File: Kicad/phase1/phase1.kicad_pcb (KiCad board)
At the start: 2 copper layers, 150.1 x 100.1 mm, 50 parts, among them Q1 IRFZ46N, Q2 IRFZ46N, Q3 IRFZ46N, Q4 IRFZ46N, Q5 IRFZ46N, Q6 IRFZ46N, U1 IR2102, U2 IR2102, U3 IR2102, U4 ACS712, U5 7805, U6 Atmega328P, Y1 Crystal

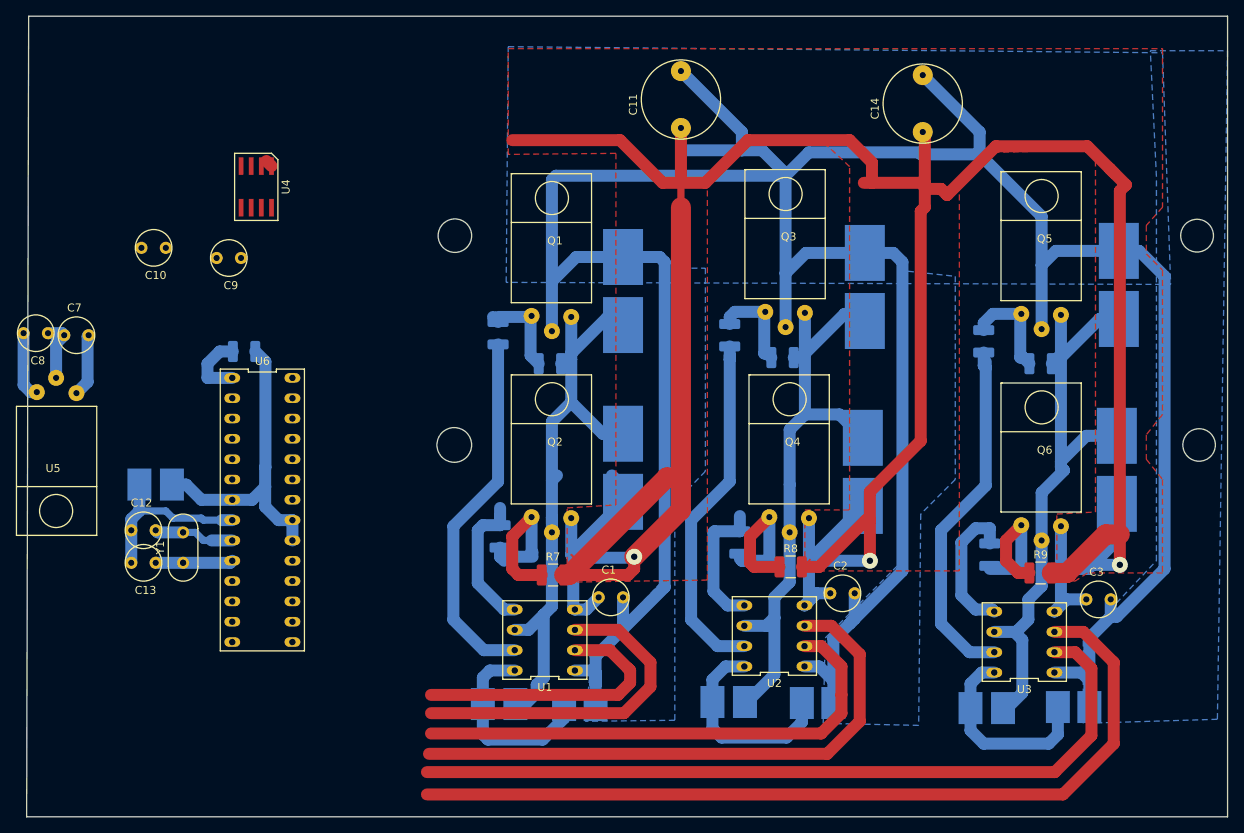
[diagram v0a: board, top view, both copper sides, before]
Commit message: .
.
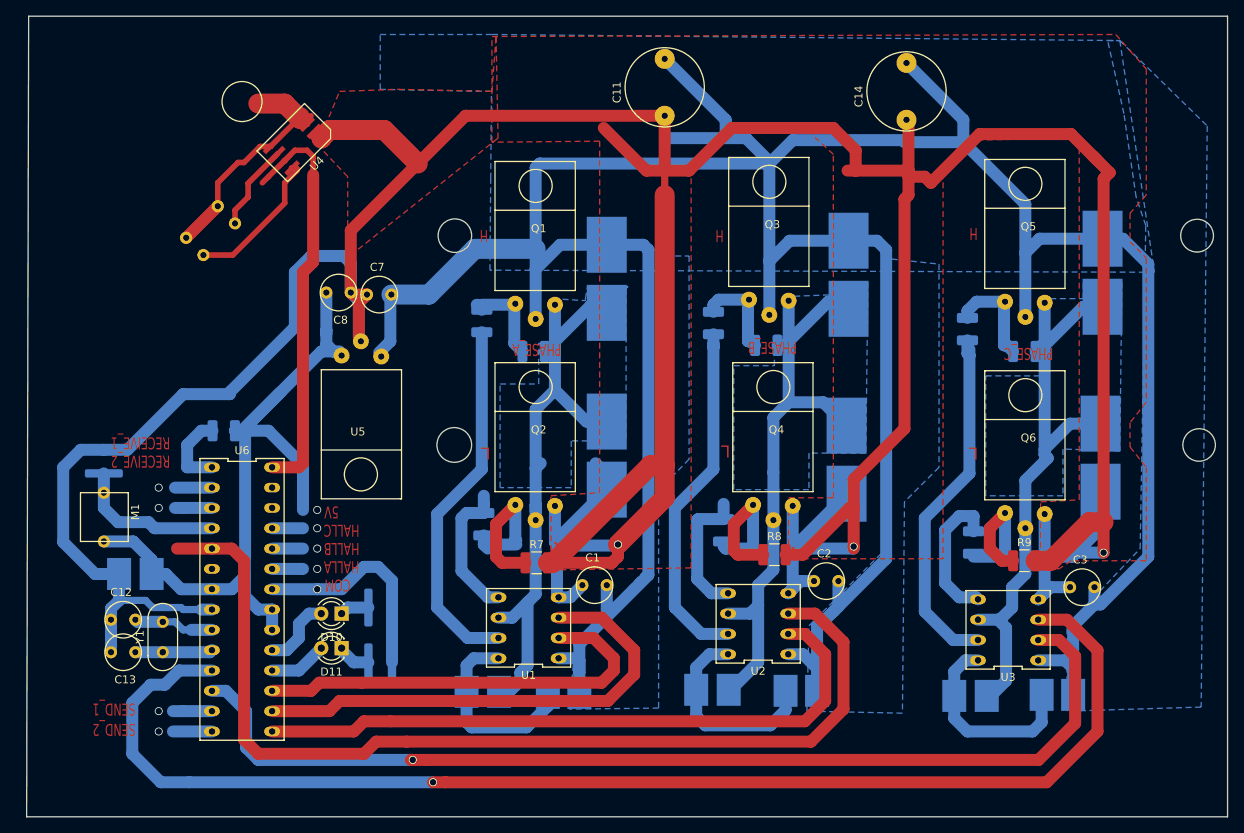
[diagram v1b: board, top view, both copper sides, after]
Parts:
- added D10: LED, LED_THT:LED_D3.0mm, F.Cu at (121.9, 87.9)
- added D11: LED, LED_THT:LED_D3.0mm, F.Cu at (121.9, 92.2)
- added M1: button, phase1:button, F.Cu at (92.2, 75.7)
- added R14: 400, Resistor_SMD:R_1218_3246Metric, B.Cu at (126.7, 87.1)
- added R15: 400, Resistor_SMD:R_1218_3246Metric, B.Cu at (126.7, 94.0)
- added R16: 10k, Resistor_SMD:R_1218_3246Metric, B.Cu at (92.2, 68.9)
- C10, C9: moved to B.Cu
- moved U5 38.4 mm to (124.5, 62.7)
- moved C7 38.2 mm to (128.0, 48.0)
- moved C8 38.2 mm to (120.1, 47.8)
- moved C10 11.9 mm to (108.5, 39.0), turned to 135 degrees
- moved C12 11.5 mm to (96.0, 88.6)
- moved C15 11.5 mm to (96.0, 83.1)
- moved Y1 11.5 mm to (99.6, 92.7)
- moved C13 11.5 mm to (93.2, 92.7)
- moved U6 11.5 mm to (109.5, 86.1)
- moved R13 10.2 mm to (107.2, 65.0)
- moved U4 7.45 mm to (116.2, 29.0), turned to 135 degrees
- moved C1 2.54 mm to (154.9, 84.3)
- moved C2 2.54 mm to (183.9, 83.8)
- moved C4 2.54 mm to (139.7, 97.5)
- moved C5 2.54 mm to (168.4, 97.3)
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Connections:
- net Net-(U6-Pad13) renamed SEND1
- net Net-(U6-Pad14) renamed SEND2
- net Net-(U6-Pad2) renamed RECEIVE1
- net Net-(U6-Pad23) renamed HALLA
- net Net-(U6-Pad24) renamed HALLB
- net Net-(U6-Pad25) renamed HALLC
- net Net-(U6-Pad3) renamed RECEIVE2
- C8 pad 1: Net-(C8-Pad1) -> 5V
- U5 pad 3: Net-(C8-Pad1) -> 5V
- U6 pad 11: Net-(U6-Pad11) -> ~LINC
- U6 pad 12: Net-(U6-Pad12) -> ~HINC
- U6 pad 15: Net-(U6-Pad15) -> ~HINB
- U6 pad 16: Net-(U6-Pad16) -> ~LINA
- U6 pad 17: Net-(U6-Pad17) -> ~HINA
- U6 pad 28: Net-(U6-Pad28) -> CURRENT
- U6 pad 4: Net-(U6-Pad4) -> BUTTON
- U6 pad 5: Net-(U6-Pad5) -> ~LINB
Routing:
- net COM: track 439.7 -> 602.5 mm
- net 5V: track 39.7 -> 97.4 mm
- net ~LINC: track 107.6 -> 161.9 mm, vias 0 -> 1
- net ~LINB: track 72.3 -> 126.1 mm
- net CURRENT: track 0.00 -> 53.5 mm
- net ~HINC: track 98.8 -> 130.1 mm, vias 0 -> 1
- net Net-(R14-Pad1): track 0.00 -> 27.1 mm, vias 0 -> 1
- net 12V: track 415.3 -> 435.7 mm
- net BUTTON: track 0.00 -> 18.9 mm
- net Net-(C9-Pad1): track 0.00 -> 18.5 mm
- net ~LINA: track 43.0 -> 61.3 mm
- net ~HINB: track 63.9 -> 82.2 mm
- net ~HINA: track 35.0 -> 53.3 mm
- net Net-(C10-Pad1): track 0.00 -> 10.9 mm
- net Net-(D10-Pad2): track 0.00 -> 9.08 mm
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- added copper zone on B.Cu, net PHASEA
- added copper zone on B.Cu, net PHASEB
- added copper zone on B.Cu, net PHASEC
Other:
- board text added: "5V"
- board text added: "COM"
- board text added: "H"
- board text added: "HALLA"
- board text added: "HALLB"
- board text added: "HALLC"
- board text added: "L"
- board text added: "PHASE_A"
- board text added: "PHASE_B"
- board text added: "PHASE_C"
- board text added: "RECEIVE_1"
- board text added: "RECEIVE_2"
- board text added: "SEND_1"
- board text added: "SEND_2"
